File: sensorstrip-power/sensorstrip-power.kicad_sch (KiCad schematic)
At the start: 11 parts, among them J1 USB_C_Receptacle_PowerOnly, J2 Conn_01x02_MountingPin, SW1 SW_DPDT_x2

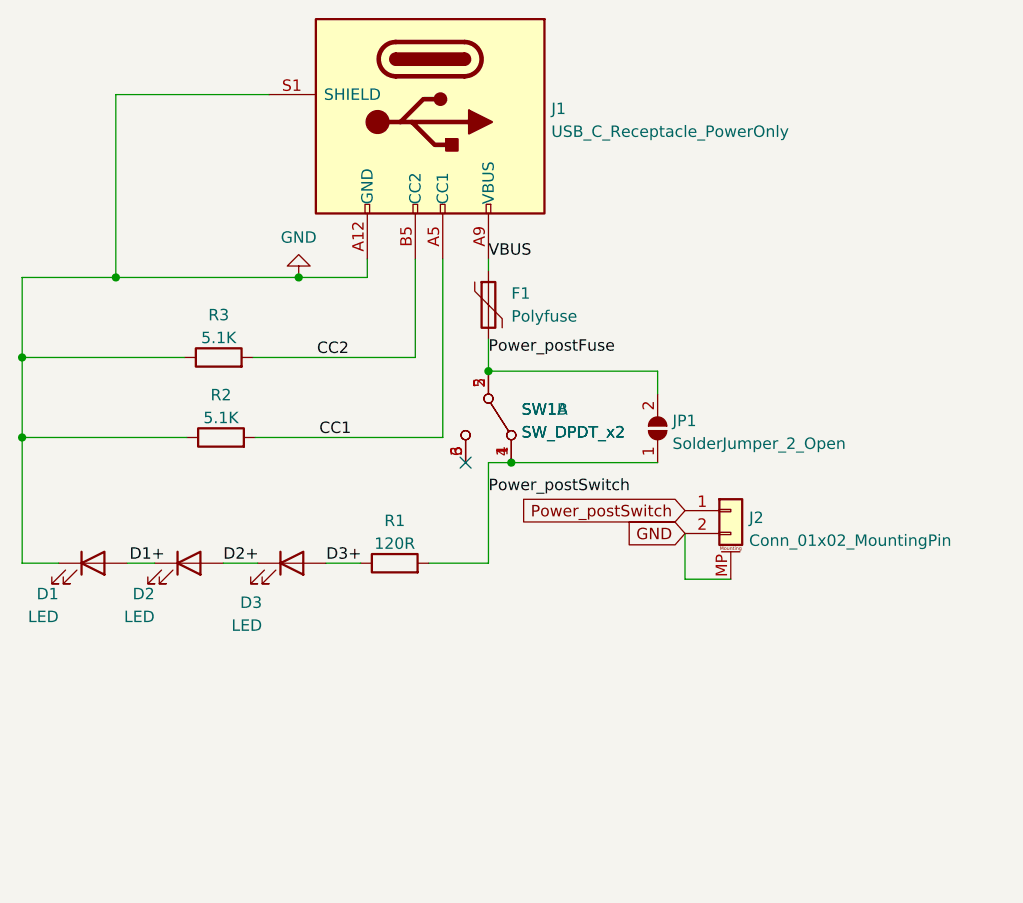
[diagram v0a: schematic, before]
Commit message: fix humongous oversight
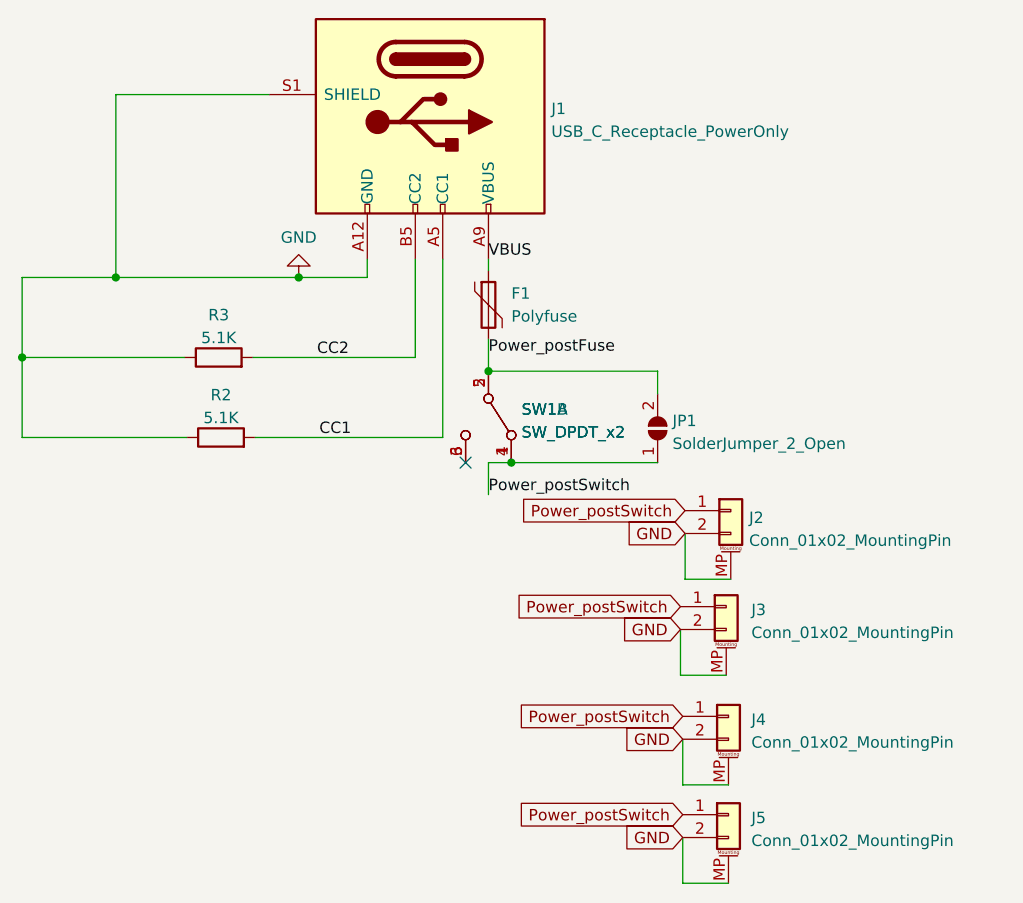
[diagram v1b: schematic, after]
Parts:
- removed D1, D2, D3: LED, sensorstrip:LED_THT-1.27mm-OrthogonalSMDAndTHT, symbol Device:LED
- removed R1: 120R, Resistor_SMD:R_0805_2012Metric_Pad1.20x1.40mm_HandSolder, symbol Device:R
- added J3, J4, J5: Conn_01x02_MountingPin, Connector_Molex:Molex_PicoBlade_53261-0271_1x02-1MP_P1.25mm_Horizontal, symbol Connector_Generic_MountingPin:Conn_01x02_MountingPin
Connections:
- net GND: now also J3.2 (Pin_2), J3.MP (MountPin), J4.2 (Pin_2), J4.MP (MountPin), J5.2 (Pin_2), J5.MP (MountPin)
- net Power_postSwitch: now also J3.1 (Pin_1), J4.1 (Pin_1), J5.1 (Pin_1)
